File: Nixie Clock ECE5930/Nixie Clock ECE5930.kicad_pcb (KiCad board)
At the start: 2 copper layers, 192 x 43.5 mm, 37 parts, among them J1 Conn_02x03_Top_Bottom, J2 USB_C_Receptacle_PowerOnly_6P, J3 Conn_01x03, SW1 SW_Push, SW2 SW_Push, SW3 SW_Push, U1 ATmega328P-P, U2 HV5622, U3 HV5622, U4 L78L05_SO8, U5 DS3231N, Y1 Crystal

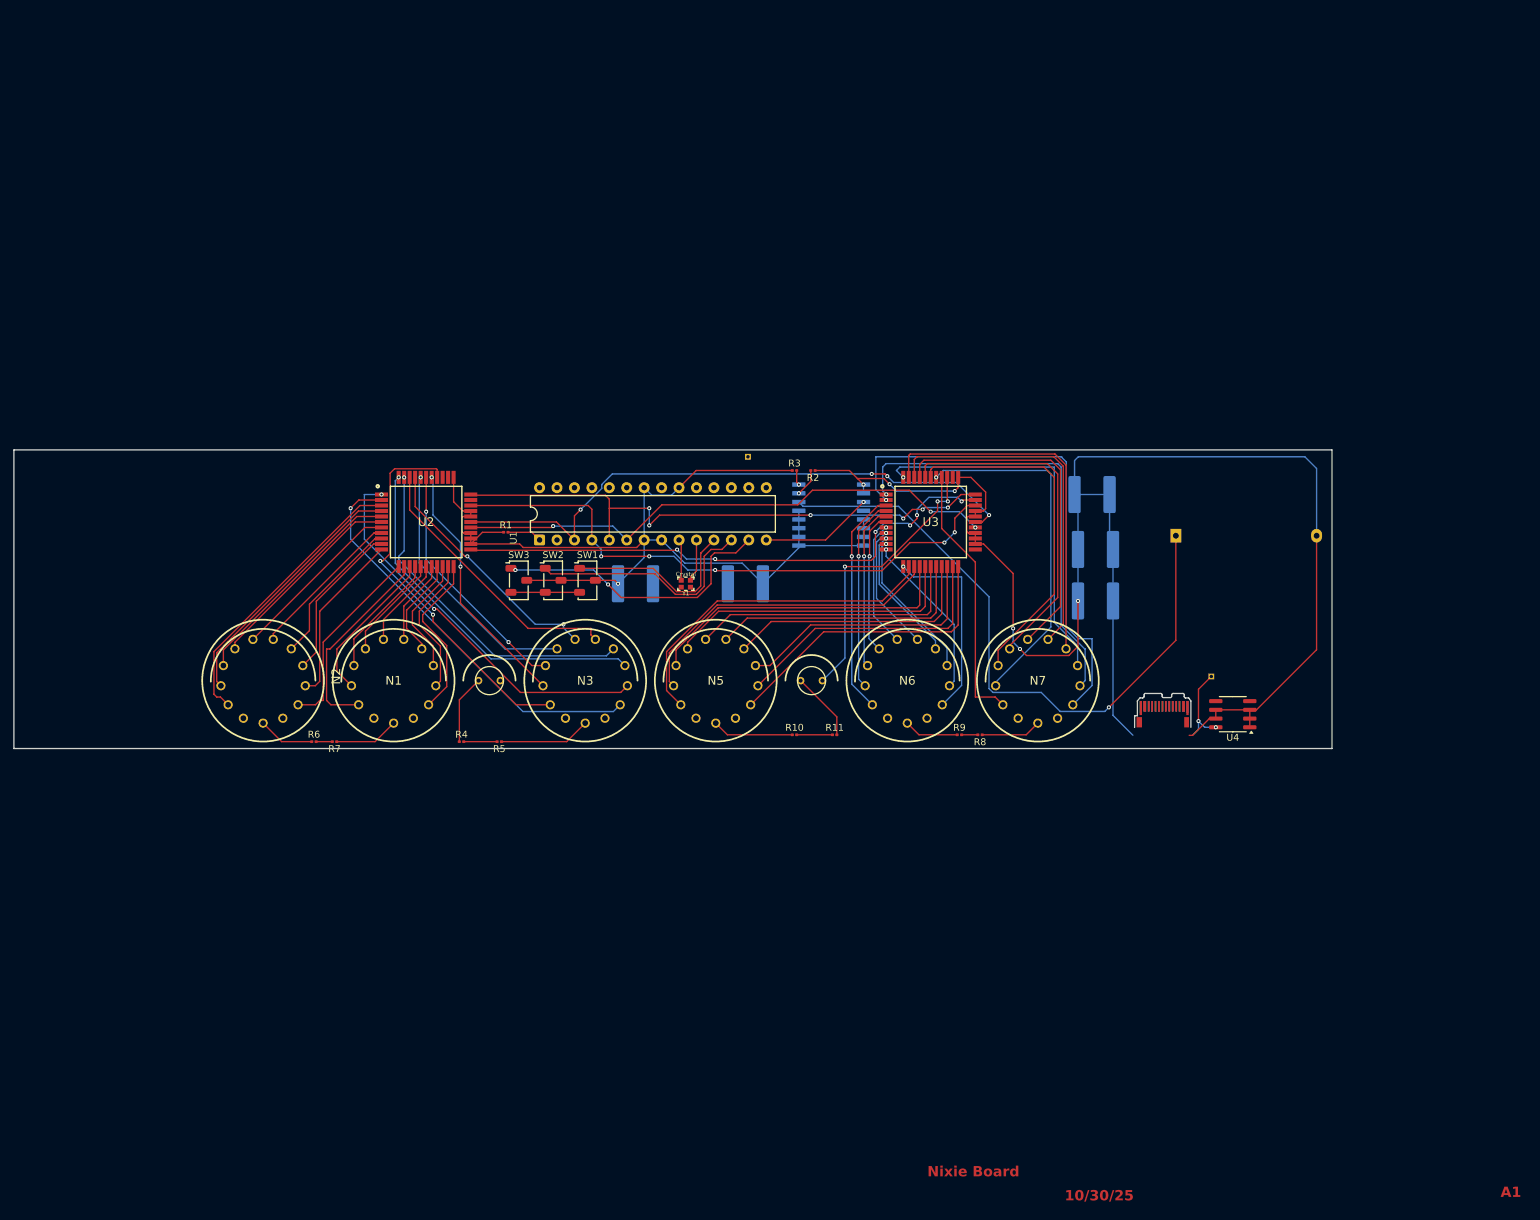
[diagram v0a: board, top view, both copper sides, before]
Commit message: rewire
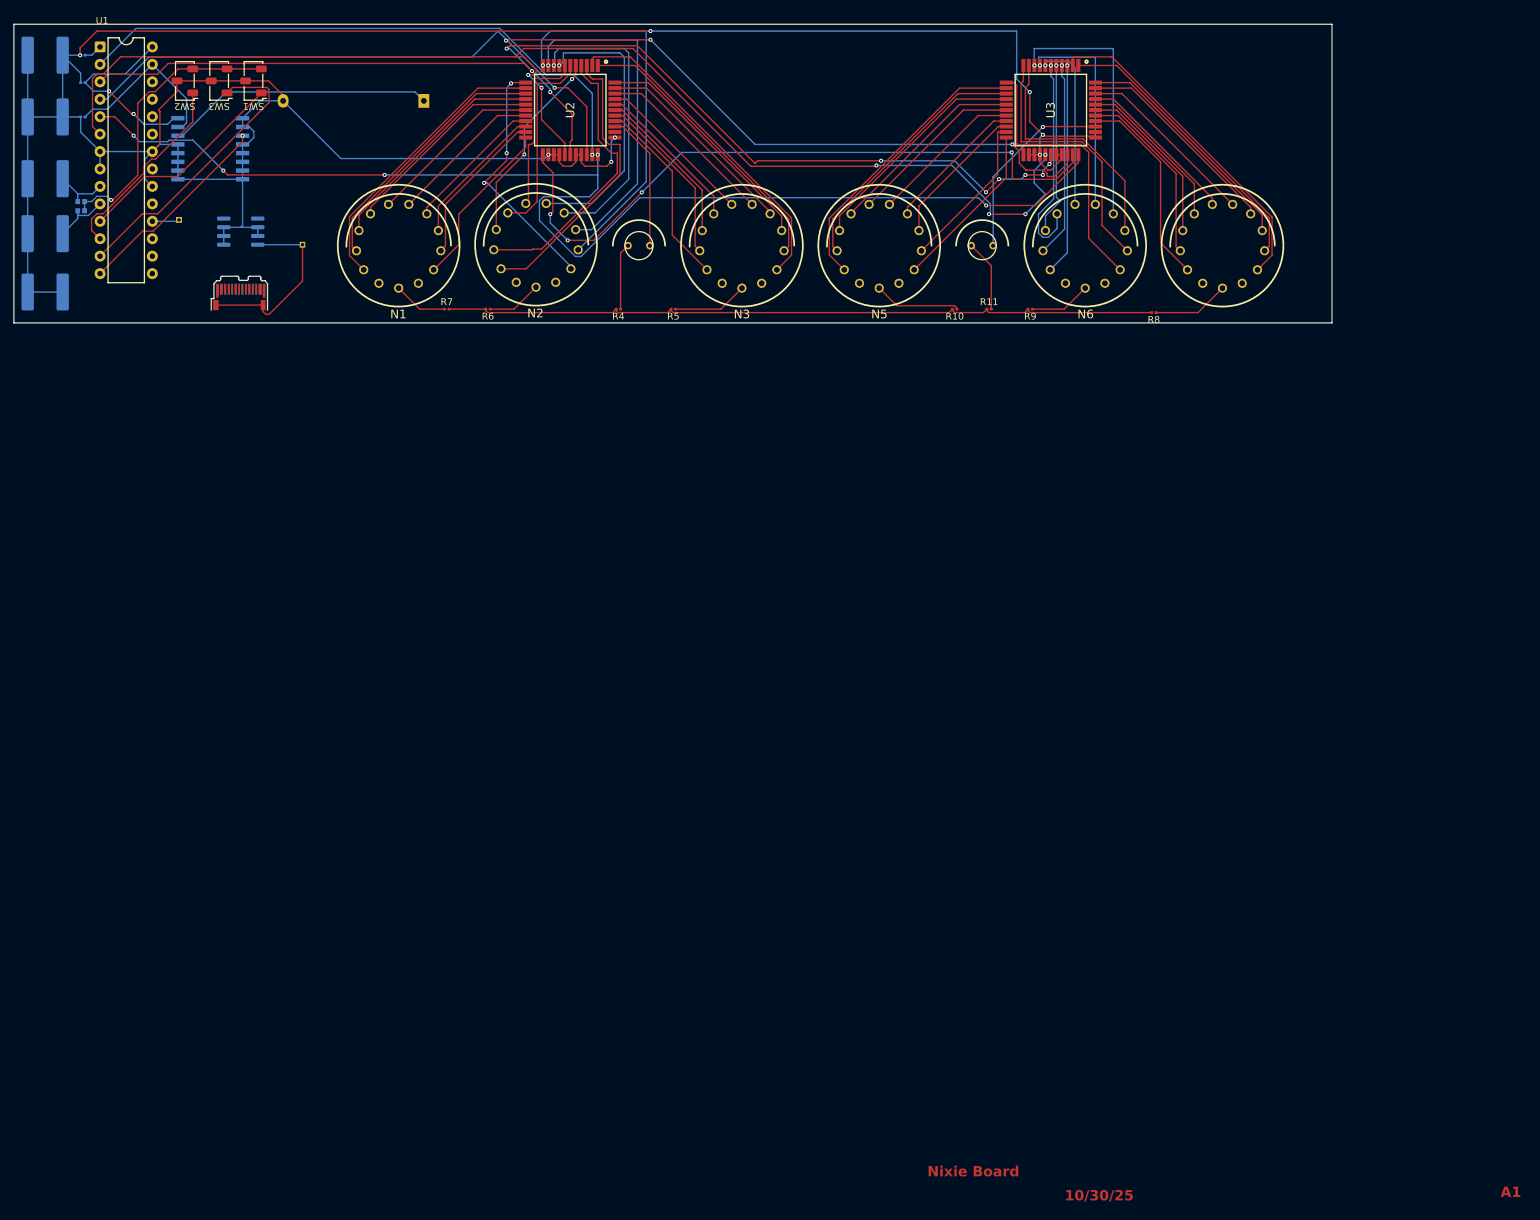
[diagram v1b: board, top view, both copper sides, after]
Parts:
- R1, R2, R3, U4, Y1: moved to B.Cu
- moved C5 169.1 mm to (58.5, 27.0), turned to 0 degrees
- moved C4 162.1 mm to (58.5, 36.0), turned to 0 degrees
- moved U4 160.7 mm to (87.0, 52.7), turned to 0 degrees
- moved C1 159.5 mm to (58.5, 61.5), turned to 0 degrees
- moved J2 147.6 mm to (87.0, 62.2)
- moved J3 146.6 mm to (96.0, 54.6)
- moved BT1 126.5 mm to (113.7, 33.7), turned to 180 degrees
- moved R2 118.2 mm to (64.0, 36.0), turned to 0 degrees
- moved R3 118.1 mm to (64.0, 31.0)
- moved C3 114.0 mm to (58.5, 53.0), turned to 0 degrees
- moved U5 105.0 mm to (82.5, 40.6)
- moved C2 104.3 mm to (58.5, 45.0)
- moved Y1 103.8 mm to (63.8, 49.0), turned to 90 degrees
- moved U1 96.2 mm to (66.5, 25.8), turned to 0 degrees
- moved R1 92.9 mm to (64.0, 27.0)
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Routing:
- net Net-(U1-PD4): track 79.7 -> 188.2 mm, vias 3 -> 6
- net Net-(U1-PD3): track 84.5 -> 181.7 mm, vias 6 -> 5
- net Net-(U1-PD2): track 85.8 -> 180.1 mm, vias 5 -> 4
- net HT: track 14.8 -> 105.3 mm
- net Net-(U1-PD1): track 87.9 -> 177.3 mm, vias 4 -> 9
- net Net-(U1-PD0): track 0.00 -> 86.7 mm, vias 0 -> 1
- net +5V: track 373.9 -> 444.0 mm, vias 7 -> 9
- net Net-(U5-Vbat): track 94.9 -> 39.0 mm, vias 1 -> 0
- net Net-(U2-HV12): track 25.3 -> 55.5 mm, vias 0 -> 1
- net Net-(U2-HV30): track 56.0 -> 27.8 mm, vias 2 -> 0
- net Net-(U3-HV27): track 50.1 -> 23.5 mm
- net Net-(U1-PC5): track 2.18 -> 28.3 mm, vias 1 -> 2
- net Net-(U3-HV28): track 50.7 -> 24.6 mm
- net Net-(U3-HV26): track 49.9 -> 23.9 mm
- net Net-(U3-HV21): track 74.3 -> 48.4 mm, vias 1 -> 0
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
